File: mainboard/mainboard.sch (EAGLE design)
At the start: 34 parts, among them U1 DWM1000, U2 ESP8266

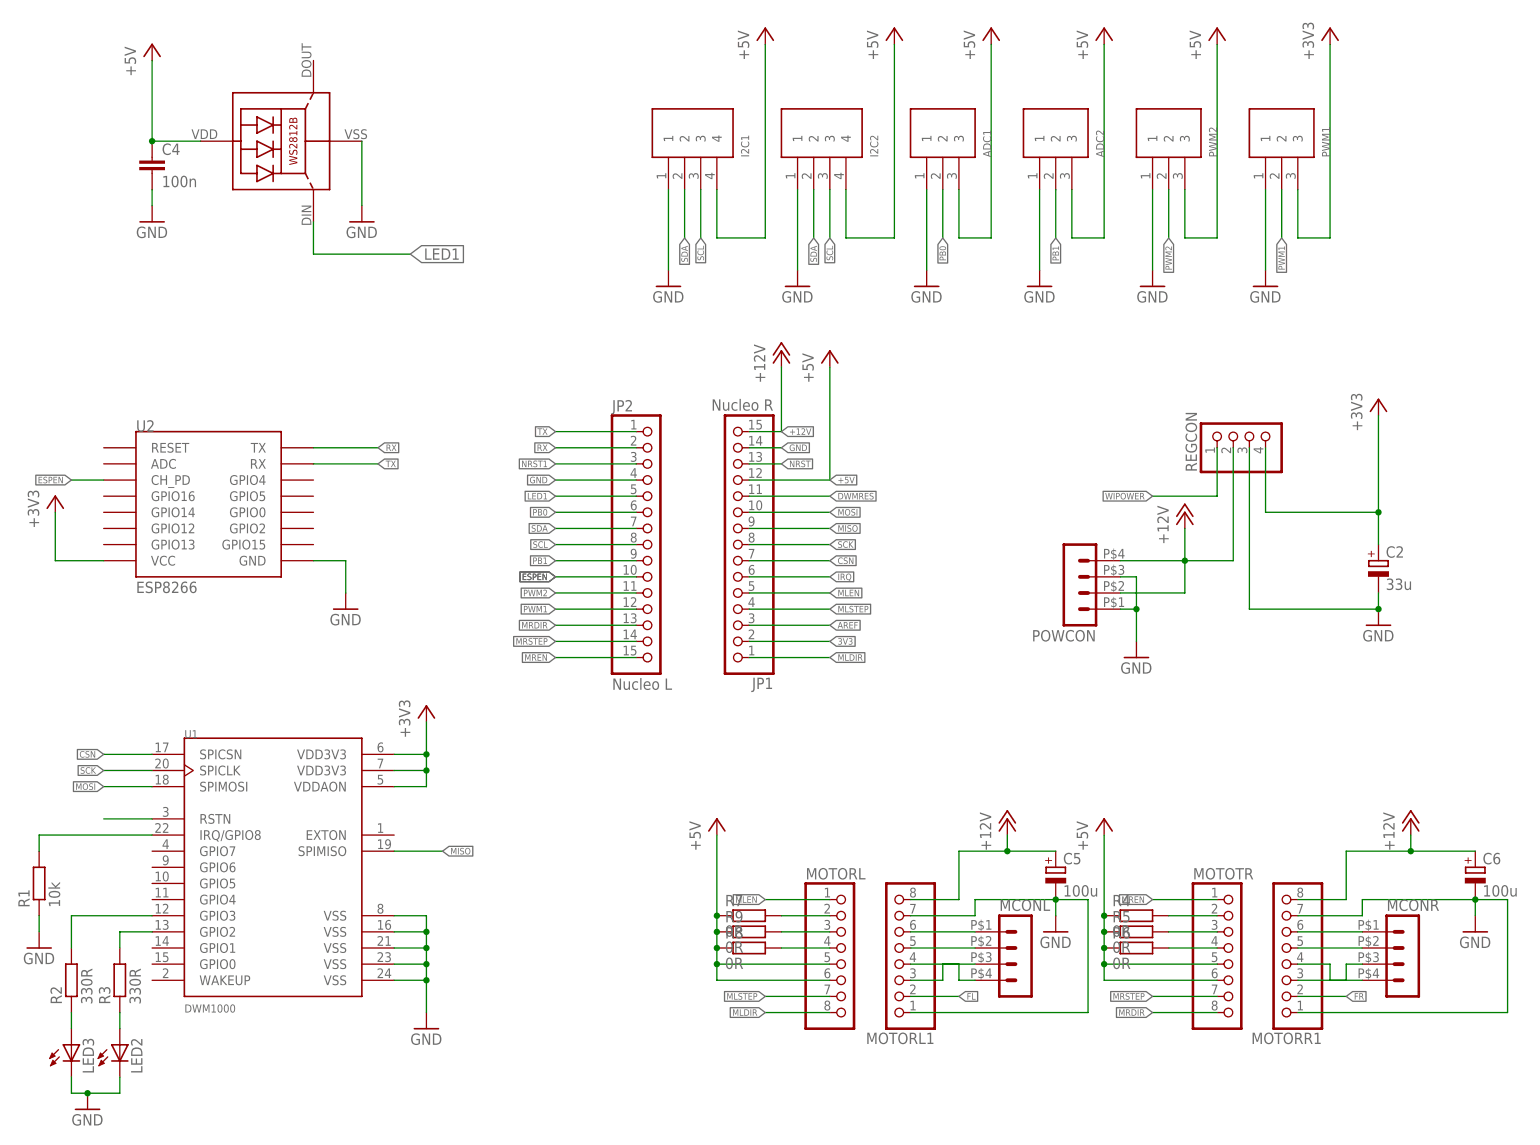
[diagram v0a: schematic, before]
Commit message: useful mods
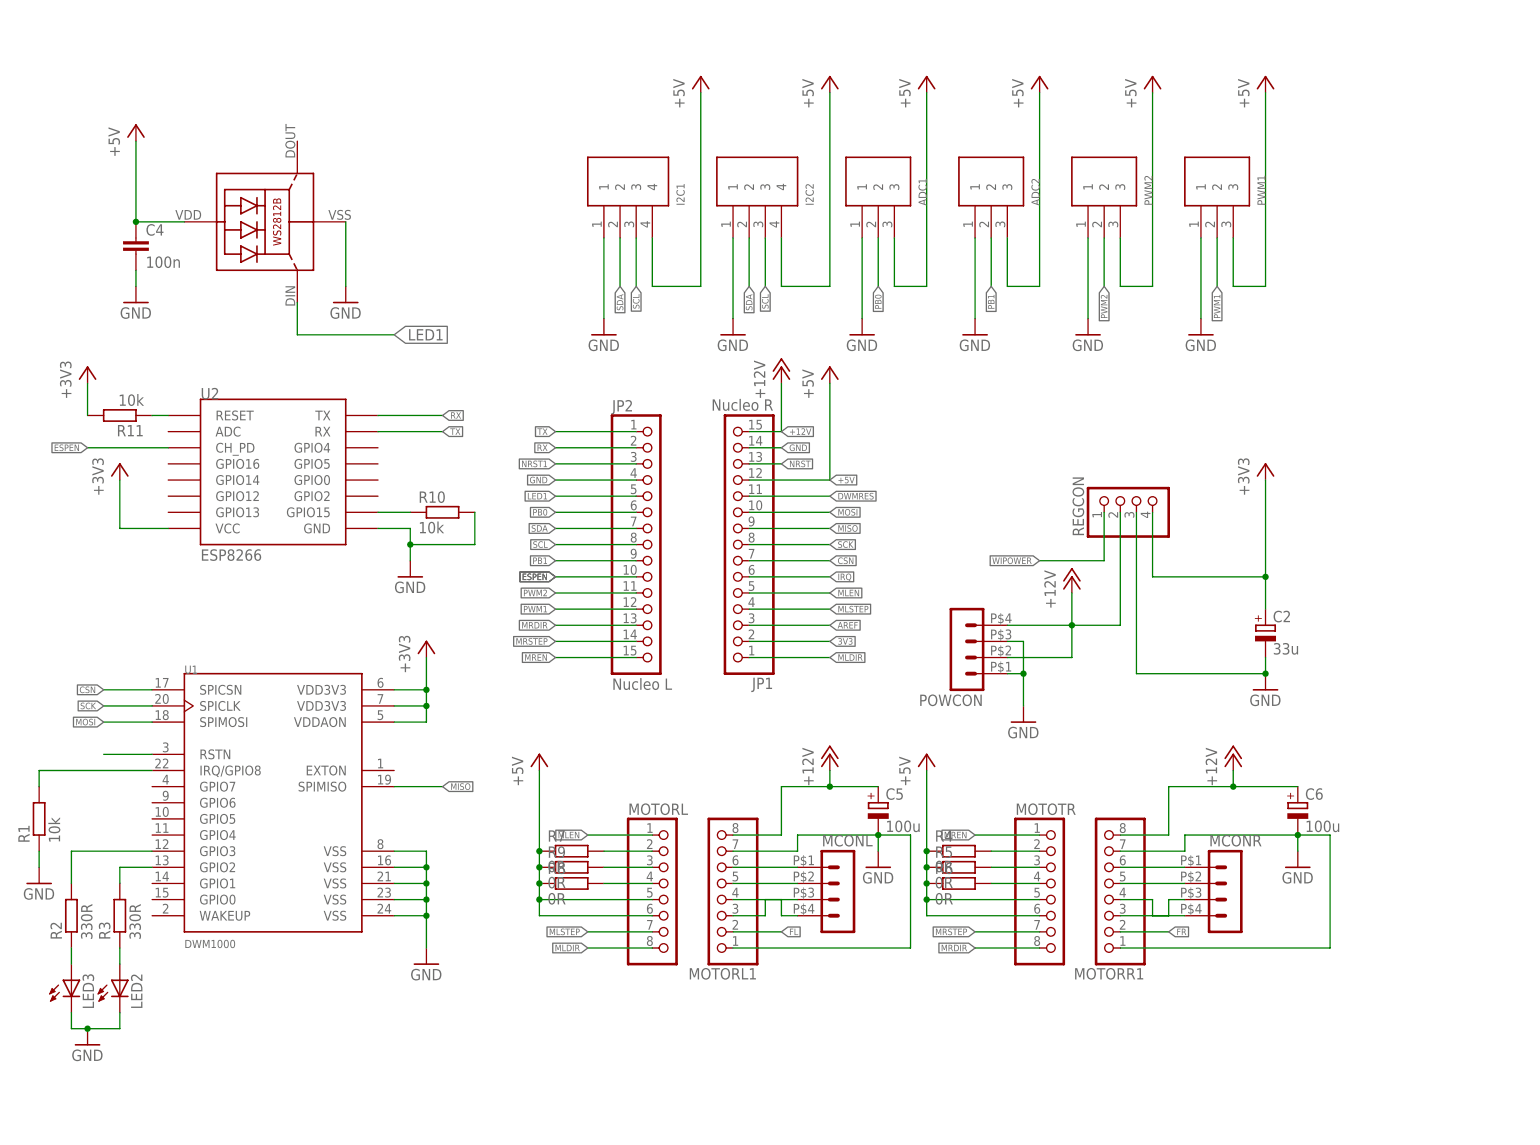
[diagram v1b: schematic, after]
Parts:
- added R10, R11: 10k, rcl:R-EU_R0603
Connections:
- new net N$16: R11.1, U2.RESET
- new net N$21: R10.1, U2.GPIO15
- net +3V3: now also R11.2; no longer PWM1.3
- net +5V: now also PWM1.3
- net GND: now also R10.2
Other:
- moved on the sheet: ADC1, ADC2, C2, C4, C5, C6, I2C1, I2C2, LED2, LED3, MCONL, MCONR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
